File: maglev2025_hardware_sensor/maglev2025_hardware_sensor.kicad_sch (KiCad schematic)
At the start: 8 parts, among them J8 Conn_01x07_MountingPin, U2 TMAG5170-Q1

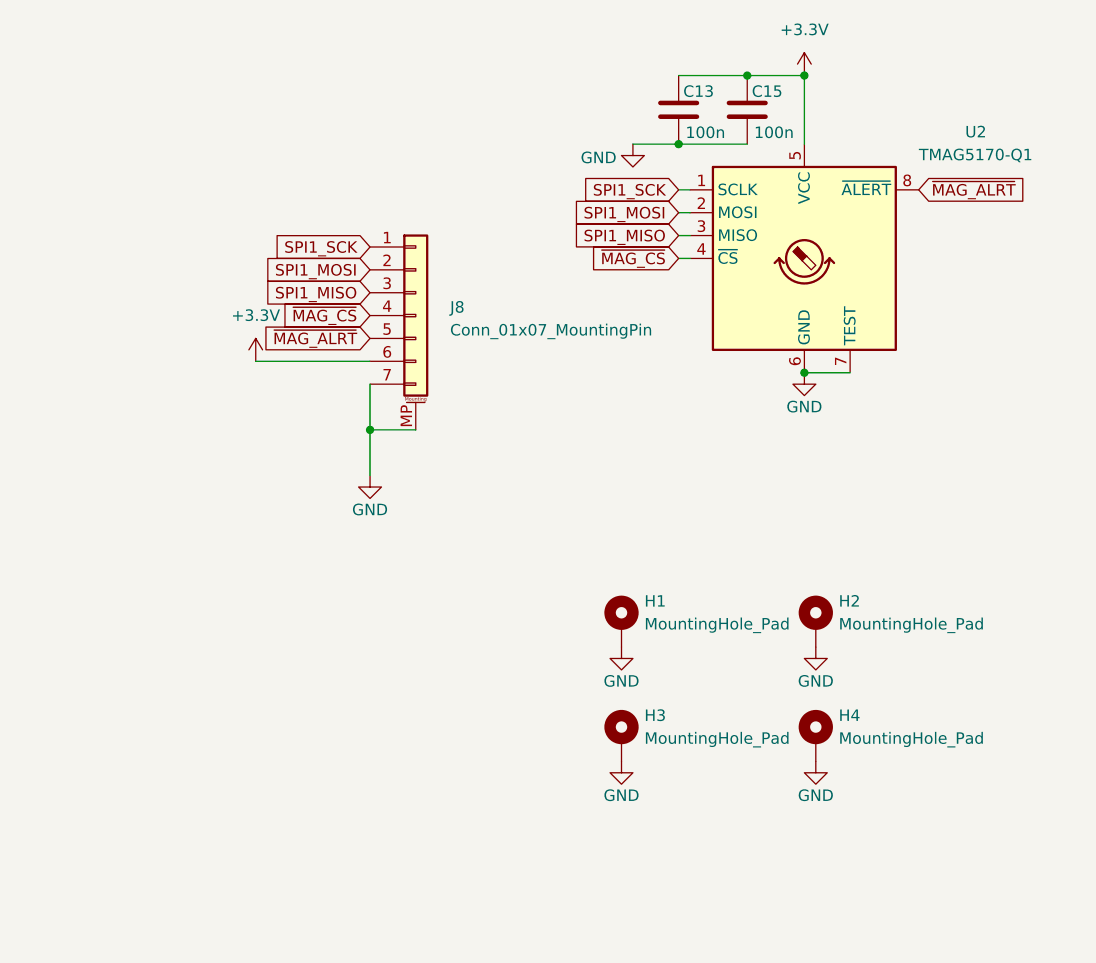
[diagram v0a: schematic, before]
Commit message: solve merge problem
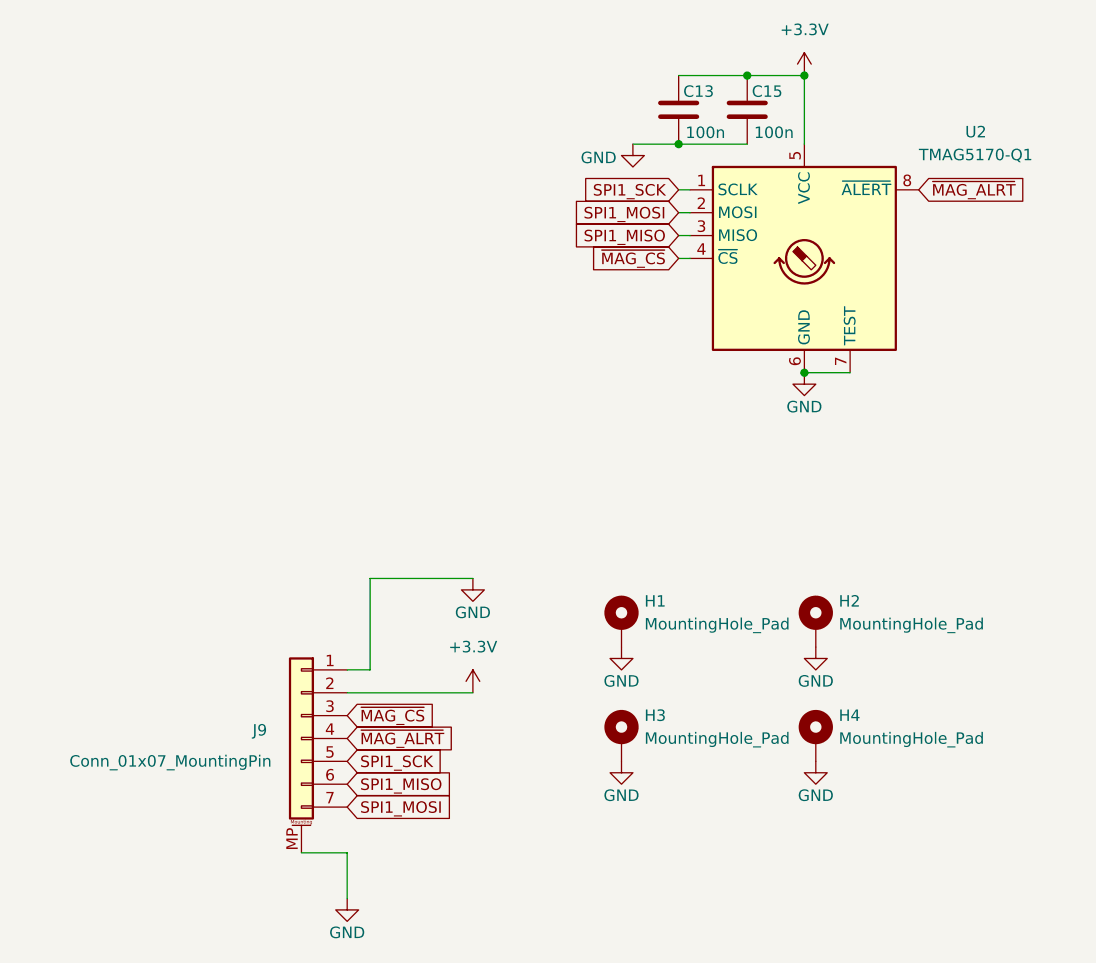
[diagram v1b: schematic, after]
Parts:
- removed J8: Conn_01x07_MountingPin, Connector_JST:JST_GH_SM07B-GHS-TB_1x07-1MP_P1.25mm_Horizontal, symbol Connector_Generic_MountingPin:Conn_01x07_MountingPin
- added J9: Conn_01x07_MountingPin, Connector_JST:JST_GH_SM07B-GHS-TB_1x07-1MP_P1.25mm_Horizontal, symbol Connector_Generic_MountingPin:Conn_01x07_MountingPin
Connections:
- net +3.3V: now also J9.2 (Pin_2)
- net GND: now also J9.1 (Pin_1), J9.MP (MountPin)
- net SPI1_MISO: now also J9.6 (Pin_6)
- net SPI1_MOSI: now also J9.7 (Pin_7)
- net SPI1_SCK: now also J9.5 (Pin_5)
- net ~{MAG_ALRT}: now also J9.4 (Pin_4)
- net ~{MAG_CS}: now also J9.3 (Pin_3)
